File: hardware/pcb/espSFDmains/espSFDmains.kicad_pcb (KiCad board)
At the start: 2 copper layers, 62.2 x 83.8 mm, 16 parts, among them J1 VDD, J2 Conn_02x10_Odd_Even, J3 Mains, J4 Mains Motor, J5 Motor, U1 WeMos_D1_mini_esp32, U2 TSR_1-2450

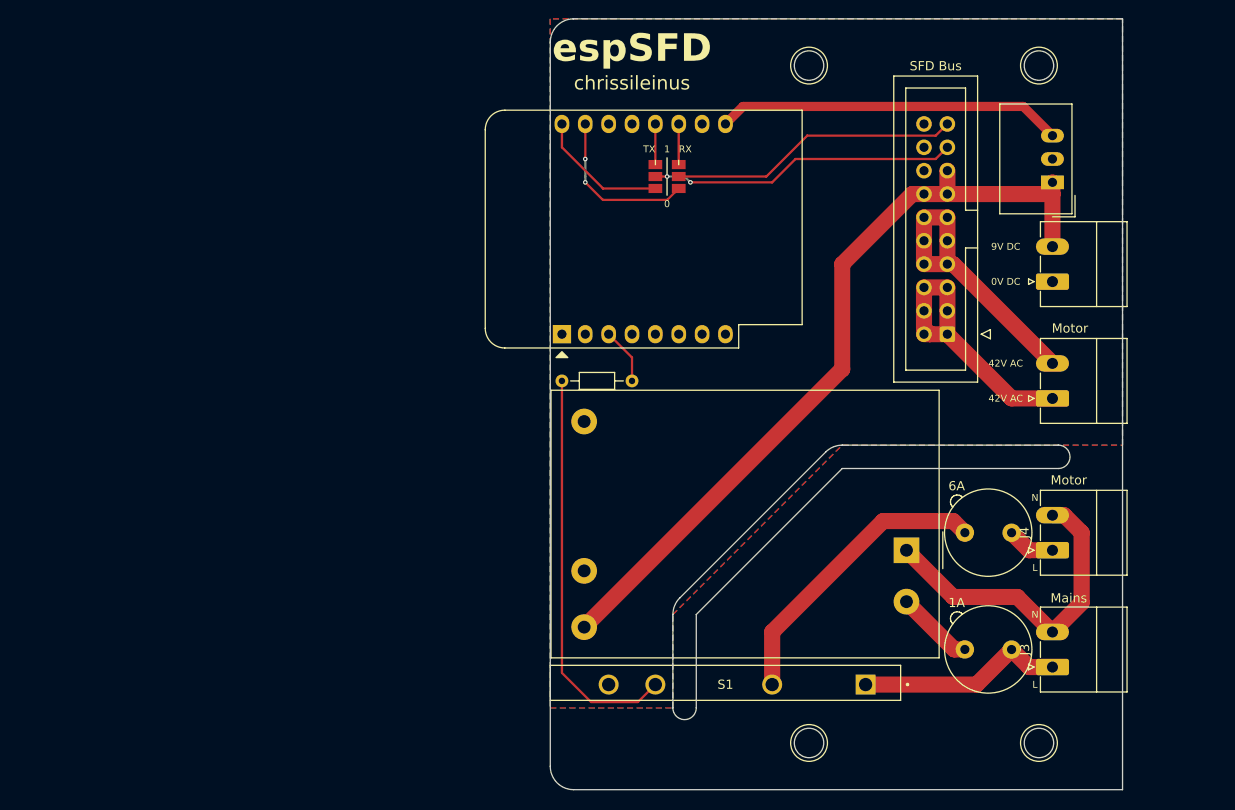
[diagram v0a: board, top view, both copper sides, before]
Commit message: PCB V1.2
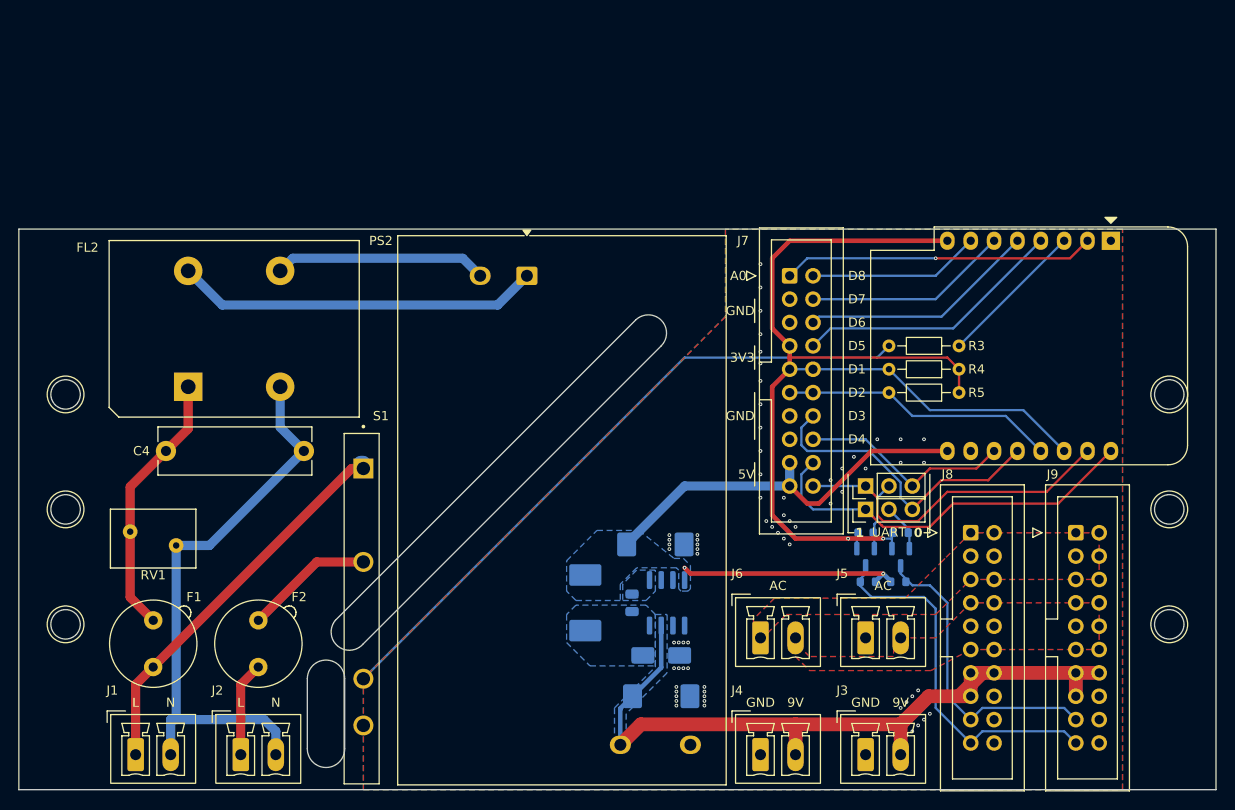
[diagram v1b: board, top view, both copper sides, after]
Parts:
- removed U1: WeMos_D1_mini_esp32, Module:WEMOS_D1_mini_light
- added C1: 15µF/50V, Capacitor_Tantalum_SMD:CP_EIA-7343-43_Kemet-X, B.Cu at (100.6, 143.8)
- added C2: 10nF/50V, Capacitor_SMD:C_0805_2012Metric, B.Cu at (97.5, 133.7)
- added C3: 68µF/16V, Capacitor_Tantalum_SMD:CP_EIA-7343-43_Kemet-X, B.Cu at (100.0, 127.3)
- added C4: 0.1uF/275Vac, Capacitor_THT:C_Rect_L16.5mm_W5.0mm_P15.00mm_MKT, F.Cu at (46.8, 117.2)
- added D1: SS14, Diode_SMD:D_SMA, B.Cu at (100.6, 139.4)
- added FL2: Choke_CommonMode_PulseElectronics_PH9455x156NL, Inductor_THT:L_CommonMode_PulseElectronics_PH9455xxx6NL_2, F.Cu at (49.2, 110.2)
- added J6: Motor, Connector_Phoenix_MC:PhoenixContact_MCV_1,5_2-G-3.81_1x02_P3.81mm_Vertical, F.Cu at (111.4, 137.5)
- added J7: Conn_02x10_Odd_Even, Connector_IDC:IDC-Header_2x10_P2.54mm_Vertical, F.Cu at (114.6, 98.1)
- added J8: Conn_02x10_Odd_Even, Connector_IDC:IDC-Header_2x10_P2.54mm_Vertical, F.Cu at (134.3, 126.0)
- added J9: Conn_02x10_Odd_Even, Connector_IDC:IDC-Header_2x10_P2.54mm_Vertical, F.Cu at (145.7, 126.0)
- added L1: 33µH, Inductor_SMD:L_Chilisin_BMRB00060650, B.Cu at (92.4, 133.7)
- added Q1: 2N7002E, Package_TO_SOT_SMD:SOT-23, B.Cu at (122.9, 128.7)
- added Q2: 2N7002H, Package_TO_SOT_SMD:SOT-23, B.Cu at (126.7, 128.7)
- added R2: 10K, Resistor_SMD:R_0603_1608Metric, B.Cu at (126.7, 126.0)
- added R3: 100R, Resistor_THT:R_Axial_DIN0204_L3.6mm_D1.6mm_P7.62mm_Horizontal, F.Cu at (133.0, 105.7)
- added R4: 4K7, Resistor_THT:R_Axial_DIN0204_L3.6mm_D1.6mm_P7.62mm_Horizontal, F.Cu at (133.0, 108.3)
- added R5: 4K7, Resistor_THT:R_Axial_DIN0204_L3.6mm_D1.6mm_P7.62mm_Horizontal, F.Cu at (133.0, 110.8)
- added R6: 10K, Resistor_SMD:R_0603_1608Metric, B.Cu at (123.1, 131.4)
- added R7: 10K, Resistor_SMD:R_0603_1608Metric, B.Cu at (126.4, 131.4)
- added RV1: 10D561K, Varistor:RV_Disc_D9mm_W6.1mm_P5mm, F.Cu at (42.9, 125.9)
- added U3: WEMOS_D1_mini, RF_Module:WEMOS_D1_mini_light, F.Cu at (149.5, 94.3)
- DRA1, DRA2: footprint Library:DINRailAdapter_3xM3_PhoenixContact_1201578 -> MountingEquipment:DINRailAdapter_3xM3_PhoenixContact_1201578
- J1: value VDD -> Mains; footprint Connector_Phoenix_MC:PhoenixContact_MC_1,5_2-G-3.81_1x02_P3.81mm_Horizontal -> Connector_Phoenix_MC:PhoenixContact_MCV_1,5_2-G-3.81_1x02_P3.81mm_Vertical
- J2: value Conn_02x10_Odd_Even -> Mains Motor; footprint Connector_IDC:IDC-Header_2x10_P2.54mm_Vertical -> Connector_Phoenix_MC:PhoenixContact_MCV_1,5_2-G-3.81_1x02_P3.81mm_Vertical
- J3: value Mains -> VDD; footprint Connector_Phoenix_MC:PhoenixContact_MC_1,5_2-G-3.81_1x02_P3.81mm_Horizontal -> Connector_Phoenix_MC:PhoenixContact_MCV_1,5_2-G-3.81_1x02_P3.81mm_Vertical
- J4: value Mains Motor -> VDD; footprint Connector_Phoenix_MC:PhoenixContact_MC_1,5_2-G-3.81_1x02_P3.81mm_Horizontal -> Connector_Phoenix_MC:PhoenixContact_MCV_1,5_2-G-3.81_1x02_P3.81mm_Vertical
- J5: footprint Connector_Phoenix_MC:PhoenixContact_MC_1,5_2-G-3.81_1x02_P3.81mm_Horizontal -> Connector_Phoenix_MC:PhoenixContact_MCV_1,5_2-G-3.81_1x02_P3.81mm_Vertical
- JP1, JP2: footprint Library:SolderJumper-3_P1.3mm_Open_Pad1.0x1.5mm no silk -> Connector_PinHeader_2.54mm:PinHeader_1x03_P2.54mm_Vertical
- PS2: value TPP-15-109-D -> HLK-30M09; footprint Converter_ACDC:Converter_ACDC_TRACO_TPP-15-1xx-D_THT -> Converter_ACDC:Converter_ACDC_Hi-Link_HLK-30Mxx
- R1: value 100R -> 10K; footprint Resistor_THT:R_Axial_DIN0204_L3.6mm_D1.6mm_P7.62mm_Horizontal -> Resistor_SMD:R_0603_1608Metric; moved to B.Cu
- U2: value TSR_1-2450 -> LM2675N-5; footprint Converter_DCDC:Converter_DCDC_TRACO_TSR-1_THT -> Package_SO:SOIC-8_3.9x4.9mm_P1.27mm; moved to B.Cu
- moved J1 112.2 mm to (43.5, 150.2), turned to 0 degrees
- moved DRA2 96.7 mm to (35.9, 123.5), turned to 90 degrees
- moved F1 93.4 mm to (45.4, 140.6), turned to 90 degrees
- moved J2 89.4 mm to (54.9, 150.2), turned to 0 degrees
- moved F2 83.2 mm to (56.8, 140.6), turned to 90 degrees
- moved U2 62.0 mm to (101.3, 133.7), turned to -90 degrees
- moved DRA1 55.1 mm to (155.9, 123.5), turned to 90 degrees
- moved PS2 50.9 mm to (86.0, 98.1), turned to -90 degrees
- moved JP2 42.8 mm to (122.9, 123.5)
- moved S1 40.4 mm to (68.1, 134.3), turned to -90 degrees
- moved JP1 39.3 mm to (122.9, 121.0)
- moved J4 38.8 mm to (111.4, 150.2), turned to 0 degrees
- moved J5 33.0 mm to (122.9, 137.5), turned to 0 degrees
- moved R1 30.3 mm to (122.9, 126.0)
- moved J3 22.4 mm to (122.9, 150.2), turned to 0 degrees
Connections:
- F1 pad 2: Net-(PS2-AC/L) -> Net-(C4-Pad1)
- J1 pad 1: VSS -> LINE
- J1 pad 2: VDD -> NEUT
- J2 pad 1: Motor N -> 230V Motor
- J2 pad 2: Motor N -> NEUT
- J3 pad 1: LINE -> VSS
- J3 pad 2: NEUT -> VDD
- J4 pad 1: 230V Motor -> VSS
- J4 pad 2: NEUT -> VDD
- JP1 pad 1: RX0 -> RX/RX0
- JP1 pad 2: RX -> Net-(JP1-C)
- JP1 pad 3: RX1 -> D4/RX1
- JP2 pad 1: TX0 -> TX/TX0
- JP2 pad 2: TX -> Net-(JP2-C)
- JP2 pad 3: TX1 -> D3/TX1
- PS2 pad 1: NEUT -> Net-(PS2-AC/L)
- PS2 pad 2: Net-(PS2-AC/L) -> Net-(PS2-AC/N)
- PS2 pad 3: unconnected-(PS2-Trim-Pad3) -> VSS
- R1 pad 1: En Motor -> Net-(JP1-C)
- R1 pad 2: Net-(S1-+LED) -> +3.3V
- U2 pad 1: VDD -> Net-(U2-CB)
- U2 pad 2: VSS -> unconnected-(U2-NC-Pad2)
- U2 pad 3: VCC -> unconnected-(U2-NC-Pad3)
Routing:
- net +3.3V: track 0.00 -> 89.4 mm, vias 0 -> 2
- net TX/TX0: track 0.00 -> 42.7 mm
- net RX/RX0: track 0.00 -> 35.7 mm
- net D3/TX1: track 0.00 -> 34.2 mm
- net A0: track 0.00 -> 34.0 mm, vias 0 -> 1
- net D1/SCL: track 0.00 -> 33.5 mm
- net Net-(PS2-AC/L): track 8.50 -> 39.7 mm
- net Motor L: track 31.1 -> 0.00 mm
- net D2/SDA: track 0.00 -> 29.9 mm
- net VCC: track 37.7 -> 67.6 mm, vias 0 -> 2
- net Motor N: track 29.8 -> 0.00 mm
- net D5: track 0.00 -> 29.5 mm
- net Net-(C4-Pad1): track 0.00 -> 29.1 mm
- net NEUT: track 35.6 -> 64.0 mm
- net Net-(S1-+LED): track 44.0 -> 72.1 mm
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- added copper zone on B.Cu, net Net-(D1-K)
- added copper zone on B.Cu, net Net-(U2-CB)
- added copper zone on B.Cu, net VCC
- added copper zone on B.Cu, net VDD
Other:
- board size 62.2 x 83.8 mm -> 130.2 x 61 mm
- board text added: "3V3"
- board text added: "5V"
- board text added: "9V"
- board text added: "A0"
- board text added: "AC"
- board text added: "D1"
- board text added: "D2"
- board text added: "D3"
- board text added: "D4"
- board text added: "D5"
- board text added: "D6"
- board text added: "D7"
- board text added: "D8"
- board text added: "GND"
- board text added: "UART"
- board text removed: "0V DC"
- board text removed: "1A"
- board text removed: "42V AC"
- board text removed: "6A"
- board text removed: "9V DC"
- board text removed: "Mains"
- board text removed: "Motor"
- board text removed: "RX"
- board text removed: "SFD Bus"
- board text removed: "TX"
- board text removed: "chrissileinus"
- board text removed: "espSFD"
